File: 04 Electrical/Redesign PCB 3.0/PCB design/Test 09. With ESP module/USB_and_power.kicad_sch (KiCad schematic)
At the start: 16 parts, among them J1 USB-C port, J3 Test connector, U2 SGM2212-3.3XKC3G/TR

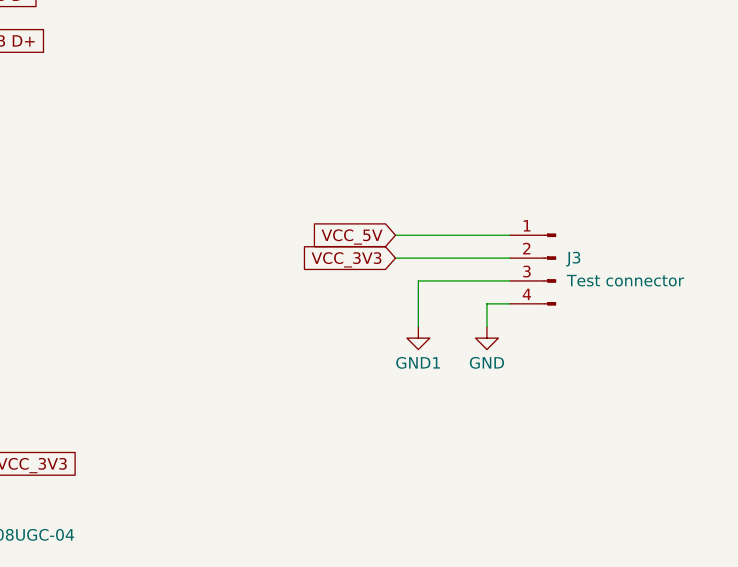
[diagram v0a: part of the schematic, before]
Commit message: Routing PCB test 9
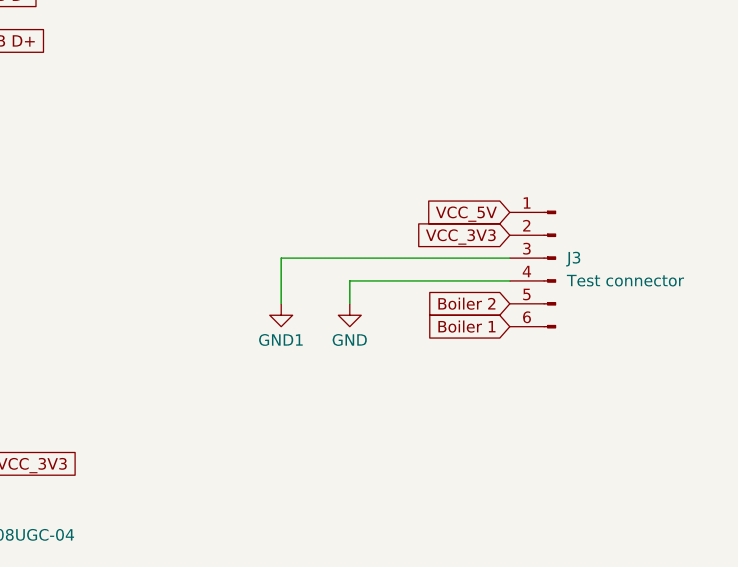
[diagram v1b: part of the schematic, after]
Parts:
- J3: footprint Project:PinHeader_1x04_P2.54mm_Horizontal -> Connector_PinHeader_2.54mm:PinHeader_1x06_P2.54mm_Vertical; symbol Connector:Conn_01x04_Pin -> Connector:Conn_01x06_Pin
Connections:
- new net Boiler 1: J3.6 (Pin_6)
- new net Boiler 2: J3.5 (Pin_5)
